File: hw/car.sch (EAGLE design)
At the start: 27 parts, among them Q1 BS170, Q2 BS170, Q3 BS170, Q4 BS170, Q5 BS170, Q6 BS170, Q7 BS170, Q8 BS170, X0 pwm_board, X1 22-23-2041, X3 22-23-2041

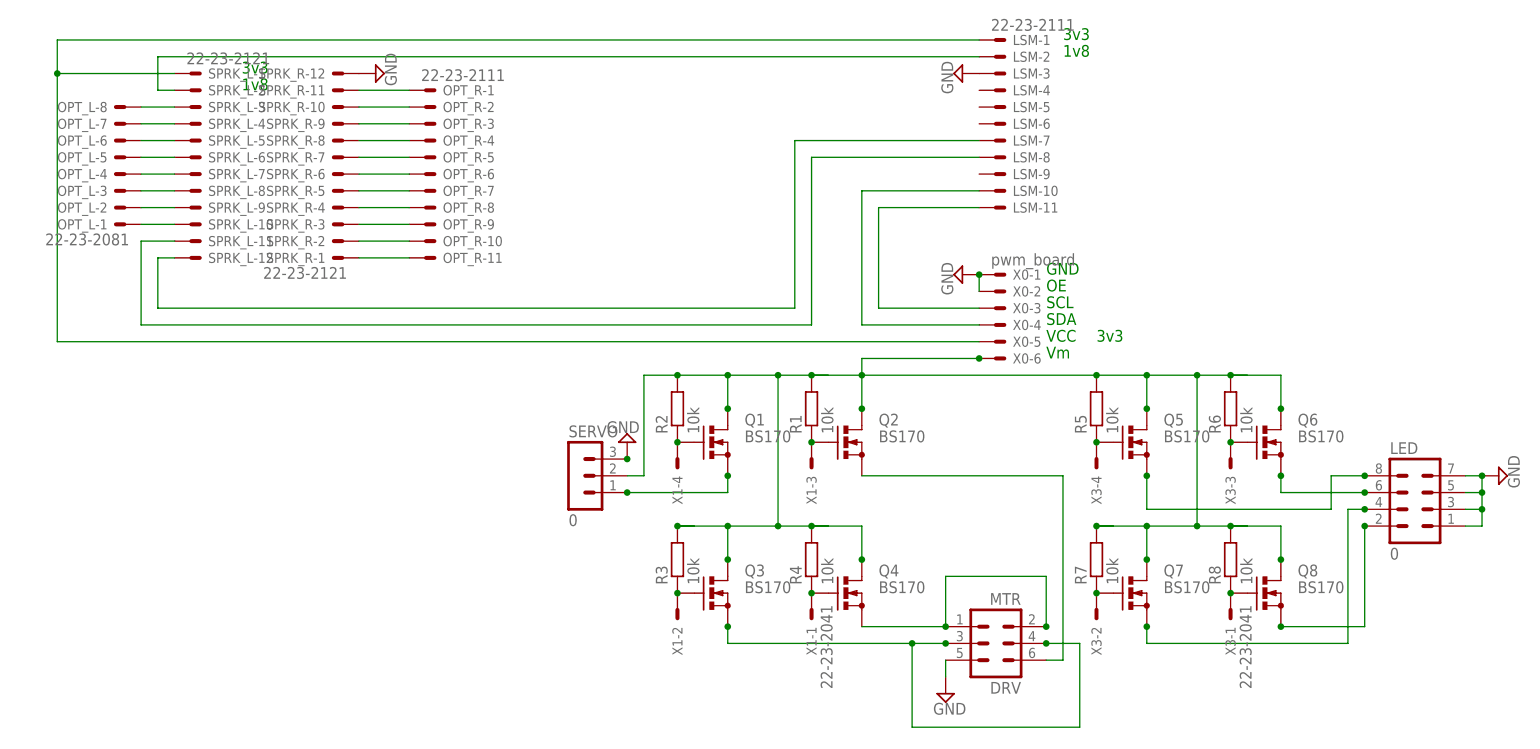
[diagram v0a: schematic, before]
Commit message: layout v1 done
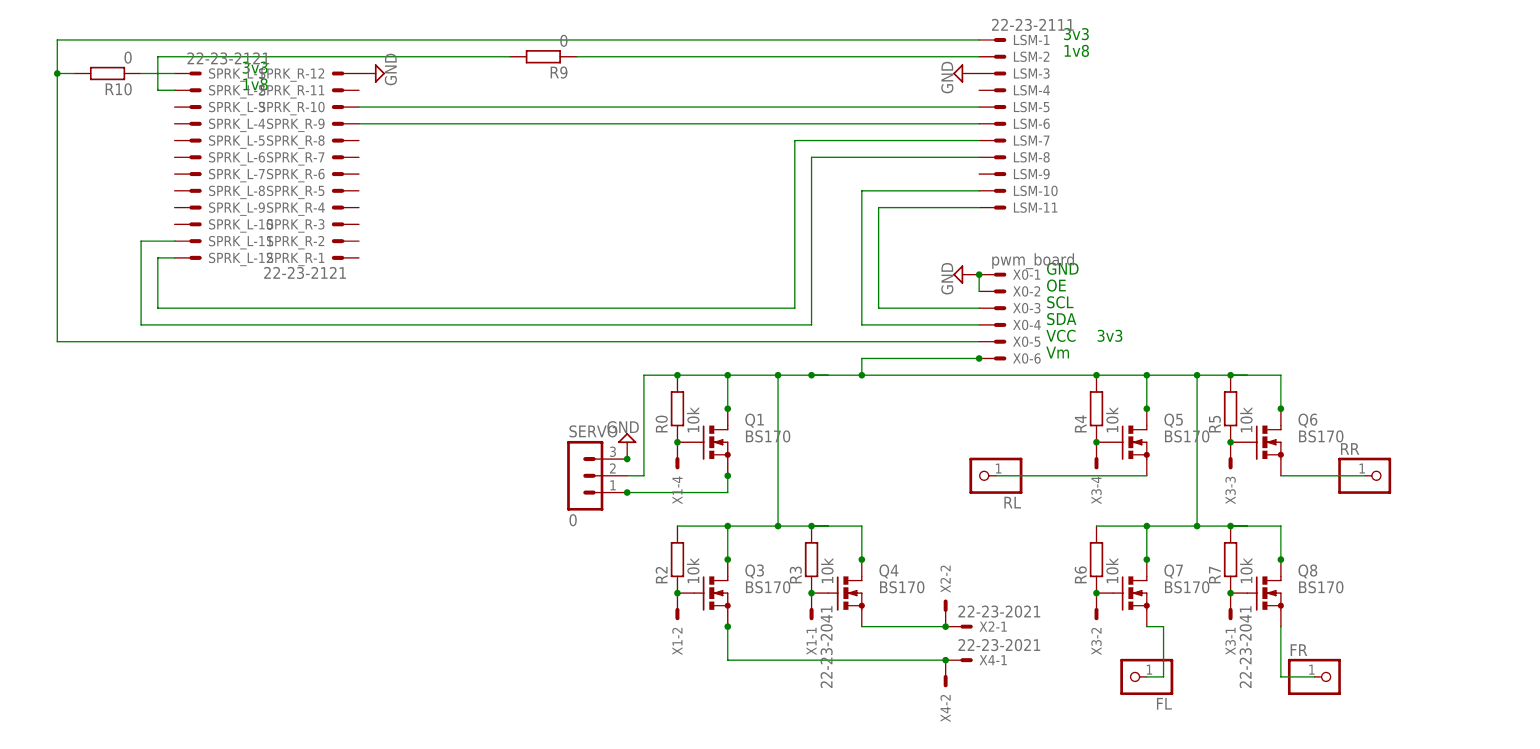
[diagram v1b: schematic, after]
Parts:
- removed DRV: MTR, con-lstb:MA03-2
- removed LED: 0, con-lstb:MA04-2
- removed OPT_L: 22-23-2081, con-molex:22-23-2081
- removed OPT_R: 22-23-2111, con-molex:22-23-2111
- removed Q2: BS170, transistor-small-signal:BS170
- removed R1, R8: 10k, rcl:R-EU_0204/2V
- added FL, FR, RL, RR: (no value), pinhead:PINHD-1X1
- added R0: 10k, rcl:R-EU_0207/10
- added R10, R9: 0, rcl:R-EU_0207/10
- added X2, X4: 22-23-2021, con-molex:22-23-2021
- R2, R3, R4, R5, R6, R7: device rcl:R-EU_0204/2V -> rcl:R-EU_0207/10
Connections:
- removed net N$15: LED.6, Q6.S
- removed net N$16: LED.8, Q5.S
- removed net N$23: OPT_L-2.S, SPRK_L-9.S
- removed net N$24: OPT_L-3.S, SPRK_L-8.S
- removed net N$25: OPT_L-4.S, SPRK_L-7.S
- removed net N$26: OPT_L-5.S, SPRK_L-6.S
- removed net N$27: OPT_L-6.S, SPRK_L-5.S
- removed net N$28: OPT_L-7.S, SPRK_L-4.S
- removed net N$29: OPT_L-8.S, SPRK_L-3.S
- removed net N$30: OPT_R-11.S, SPRK_R-1.S
- removed net N$31: OPT_R-10.S, SPRK_R-2.S
- removed net N$32: OPT_R-9.S, SPRK_R-3.S
- removed net N$33: OPT_R-8.S, SPRK_R-4.S
- removed net N$34: OPT_R-7.S, SPRK_R-5.S
- removed net N$35: OPT_R-6.S, SPRK_R-6.S
- removed net N$36: OPT_R-5.S, SPRK_R-7.S
- removed net N$37: OPT_R-4.S, SPRK_R-8.S
- removed net N$40: OPT_R-1.S, SPRK_R-11.S
- removed net N$41: DRV.6, Q2.S
- new net 1V8: LSM-2.S, R9.1
- new net V3V3: LSM-1.S, R10.2, X0-5.S
- net GND: no longer DRV.5, LED.1, LED.3, LED.5, LED.7
- net N$1: now also R0.1; no longer R2.1
- net N$10: now also R4.1; no longer R5.1
- net N$11: now also R5.1; no longer R6.1
- net N$12: now also R6.1; no longer R7.1
- net N$13: now also R7.1; no longer R8.1
- net N$14: now also FL.1; no longer LED.4
- net N$17: now also R9.2; no longer LSM-2.S
- net N$2: now also Q4.S, X2-1.S, X2-2.S; no longer Q2.G, R1.1, X1-3.S
- net N$22: now also R10.1, SPRK_L-1.S; no longer OPT_L-1.S, SPRK_L-10.S
- net N$3: now also R2.1; no longer R3.1
- net N$38: now also LSM-6.S; no longer OPT_R-3.S
- net N$39: now also LSM-5.S; no longer OPT_R-2.S
- net N$4: now also R3.1; no longer R4.1
- net N$6: now also Q5.S, RL.1; no longer DRV.1, DRV.2, Q4.S
- net N$7: now also Q6.S, RR.1; no longer DRV.3, DRV.4, Q3.S
- net N$8: now also Q3.S, X4-1.S, X4-2.S; no longer LSM-1.S, SPRK_L-1.S, X0-5.S
- net N$9: now also FR.1; no longer LED.2
- net VM: now also R0.2; no longer Q2.D, R1.2, R8.2
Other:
- moved on the sheet: R2, R3, R4, R5, R6, R7
